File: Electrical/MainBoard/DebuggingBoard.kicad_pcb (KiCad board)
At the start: 6 copper layers, 90 x 90 mm, 167 parts, among them J1 Barrel_Jack_Switch, Q1 AO3401A, SW1 SW_SPDT, U1 CH224K, U10 FFC2B28-24-G, U11 SM08B-PASS-TBT(LF)(SN), U12 SM05B-PASS-TBT(LF)(SN), U13 SM02B-PASS-TBT(LF)(SN), U14 SM08B-PASS-TBT(LF)(SN), U15 SM05B-PASS-TBT(LF)(SN), U16 SM05B-PASS-TBT(LF)(SN), U17 SM05B-PASS-TBT(LF)(SN), U18 SM03B-PASS-TBT(LF)(SN)_C412099, U19 SM03B-PASS-TBT(LF)(SN)_C412099, U2 STM32H723VGTx, U20 SM06B-PASS-TBT(LF)(SN), U21 SM06B-PASS-TBT(LF)(SN), U22 SM09B-PASS-TBT(LF)(SN), U23 SM05B-PASS-TBT(LF)(SN), U24 SM04B-PASS-TBT(LF)(SN), U25 PJ-002BH, U26 SM06B-PASS-TBT(LF)(SN), U3 APS6404L-3SQR-ZR, U4 USB3300-EZK, U5 TPS65131RGE, U6 TPS2121RUXR, U7 TPS7A9401DSCR, U8 LM61460AASQRJRRQ1, U9 S5B-ZR-SM4A-TF(LF)(SN), Y1 X322525MOB4SI, Y2 X322524MOB4SI

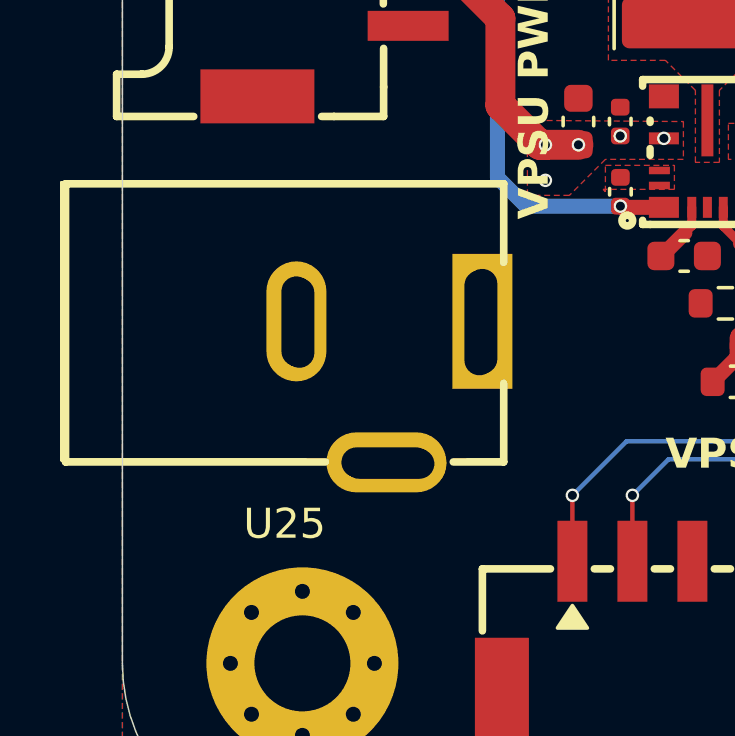
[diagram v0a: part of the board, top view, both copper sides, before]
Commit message: software unit testing
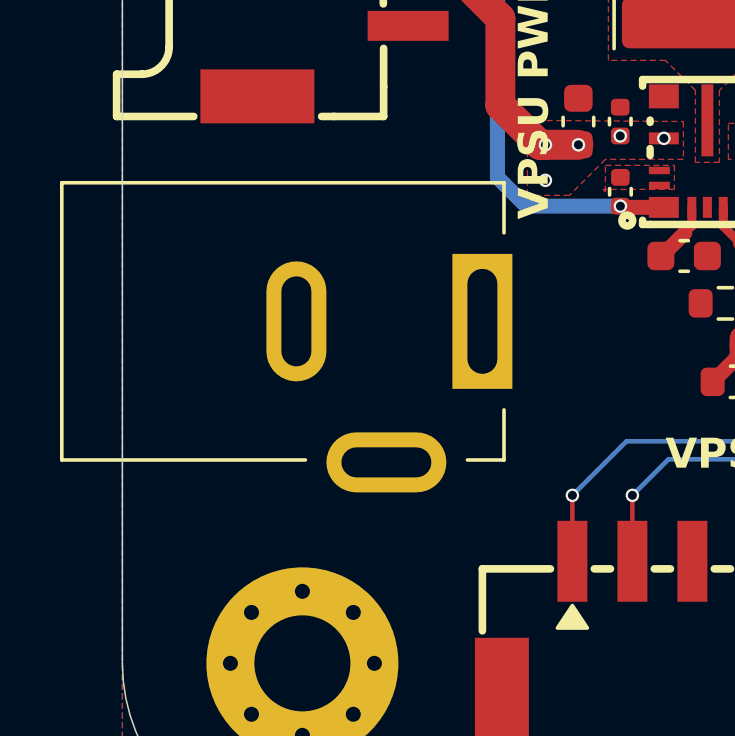
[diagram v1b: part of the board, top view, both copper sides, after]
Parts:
- removed U25: PJ-002BH, JLC_PARTS:DC-IN-TH_PJ-002BH
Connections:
- C66 pad 2: +5V -> Net-(U8-SW)
